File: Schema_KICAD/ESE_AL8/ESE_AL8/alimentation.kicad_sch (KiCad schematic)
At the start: 26 parts, among them IC1 MP1475SGJ-P, J6 Batterie, SW2 ON/OFF, U2 BUxxSD5

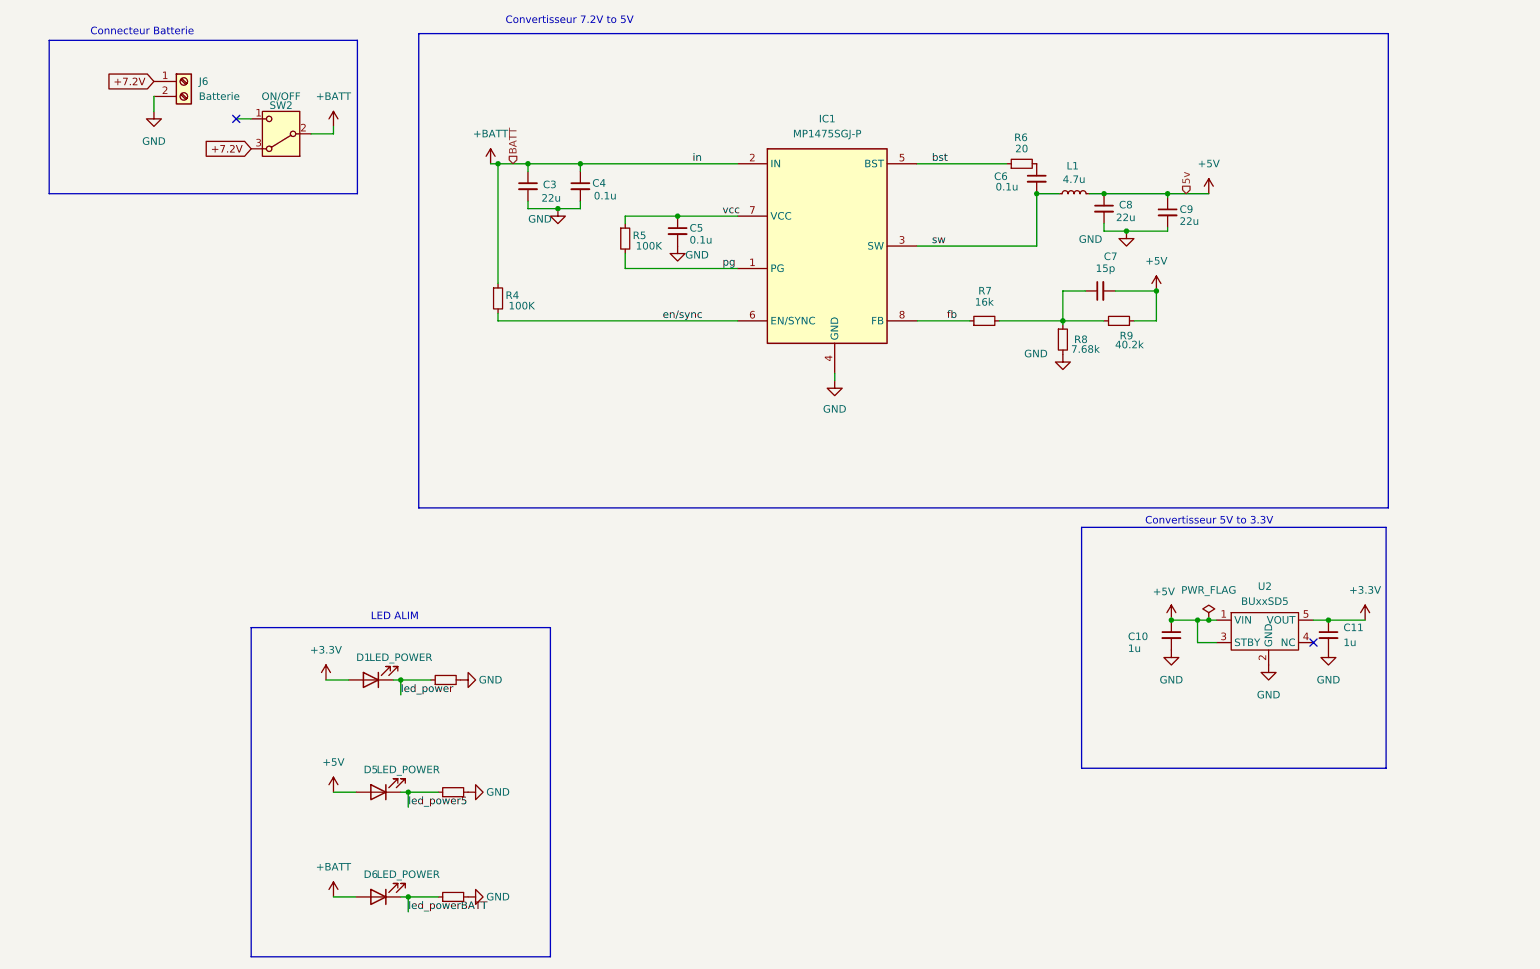
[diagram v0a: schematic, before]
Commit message: le bon ioc
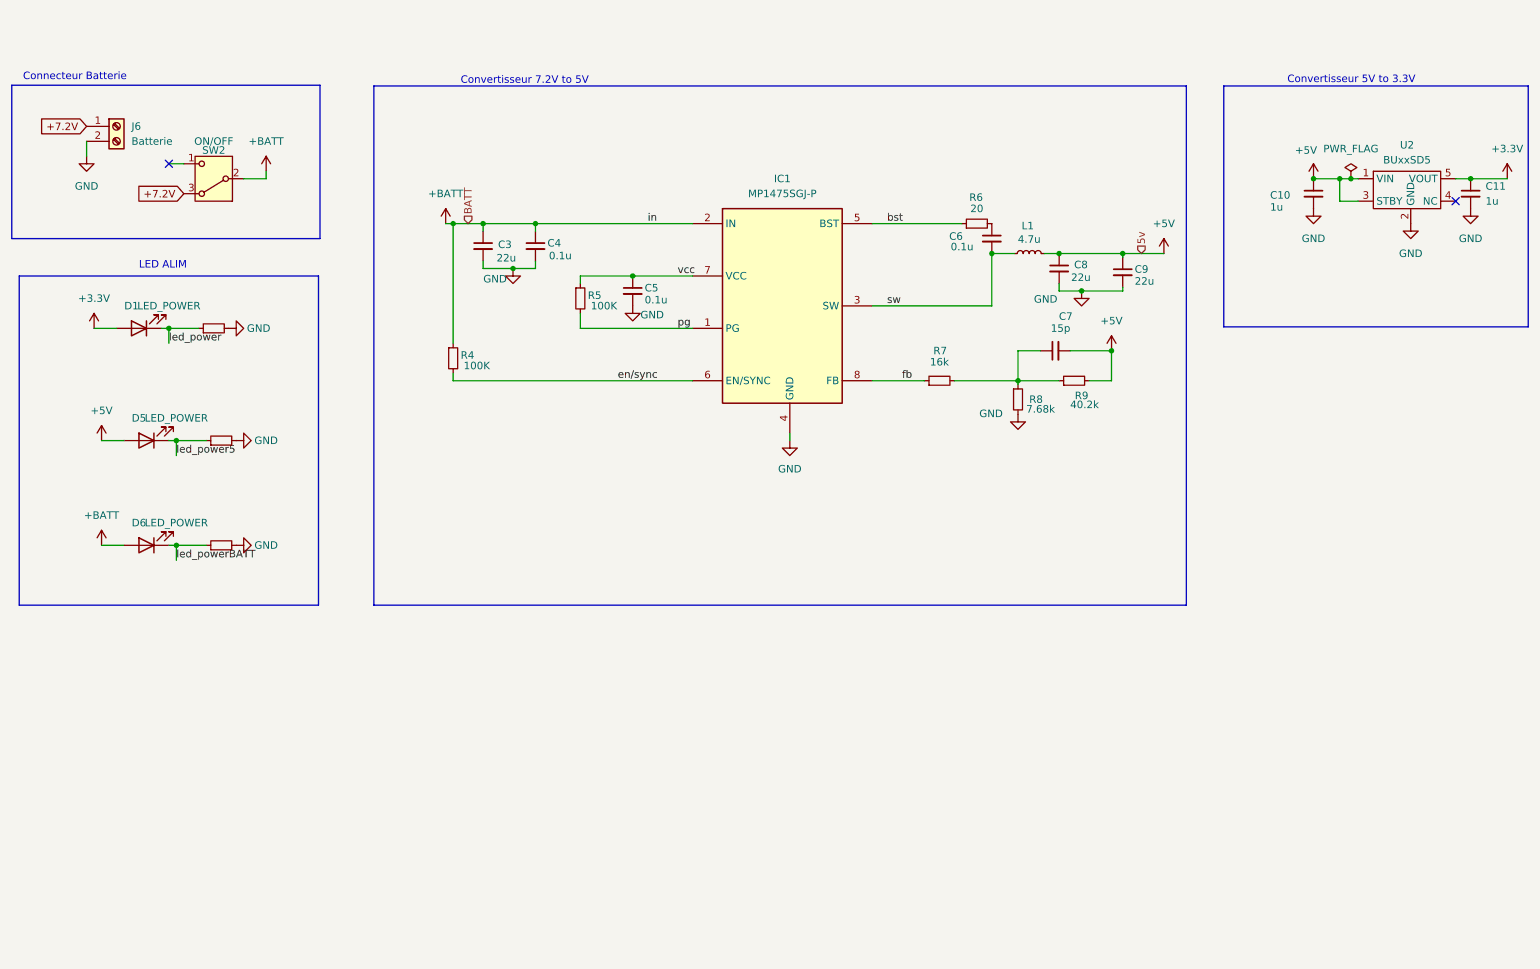
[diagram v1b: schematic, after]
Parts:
- R14: value 680 -> 2.5
- R15: value 680 -> 4.2
- R3: value 680 -> 1k
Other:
- moved on the sheet: C10, C11, C3, C4, C5, C6, C7, C8, C9, D1, D5, D6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
